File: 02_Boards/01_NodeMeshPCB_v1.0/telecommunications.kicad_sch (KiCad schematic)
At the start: 0 parts

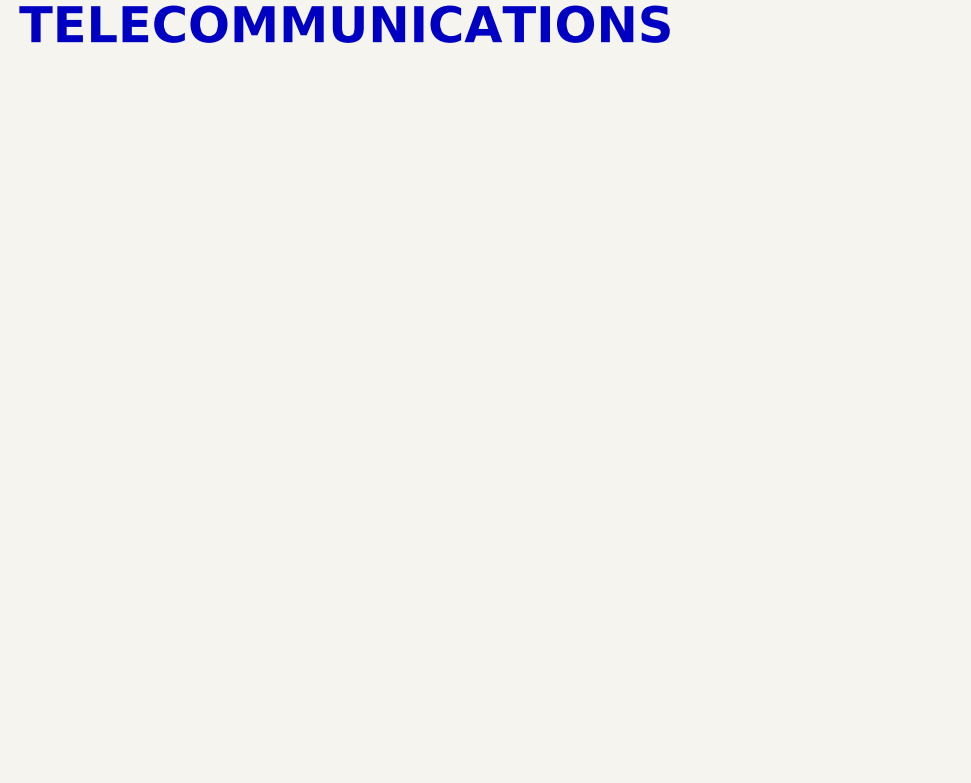
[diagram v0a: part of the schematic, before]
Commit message: ht-ra62 schematic
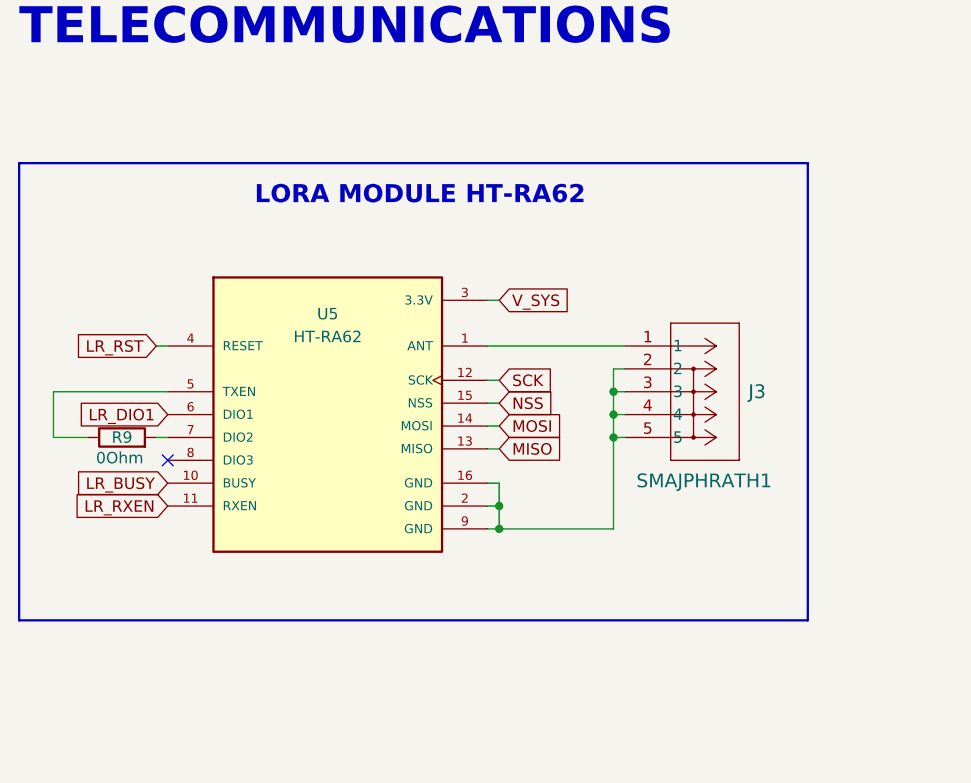
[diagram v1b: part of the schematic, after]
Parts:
- added J3: SMAJPHRATH1, CONN_SMA-J-P-H-RA-TH1_SAI, symbol SMAJPHRATH1:SMA-J-P-H-RA-TH1
- added R9: 0Ohm, symbol Device:R
- added U5: HT-RA62, symbol HT-RA62:HT-RA62
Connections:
- new net: R9.1, U5.5 (TXEN)
- new net: R9.2, U5.7 (DIO2)
- new net: J3.1, U5.1 (ANT)
- new net: J3.2, J3.3, J3.4, J3.5, U5.16 (GND), U5.2 (GND), U5.9 (GND)
- new net LR_BUSY: U5.10 (BUSY)
- new net LR_DIO1: U5.6 (DIO1)
- new net LR_RST: U5.4 (RESET)
- new net LR_RXEN: U5.11 (RXEN)
- new net MISO: U5.13 (MISO)
- new net MOSI: U5.14 (MOSI)
- new net NSS: U5.15 (NSS)
- new net SCK: U5.12 (SCK)
- new net V_SYS: U5.3 (3.3V)
- no-connect marks 0 -> 1
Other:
- note added: "LORA MODULE HT-RA62"
